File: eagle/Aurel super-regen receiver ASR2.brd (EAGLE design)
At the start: 43.2 x 25.4 mm, 15 parts, among them T1 BF247B

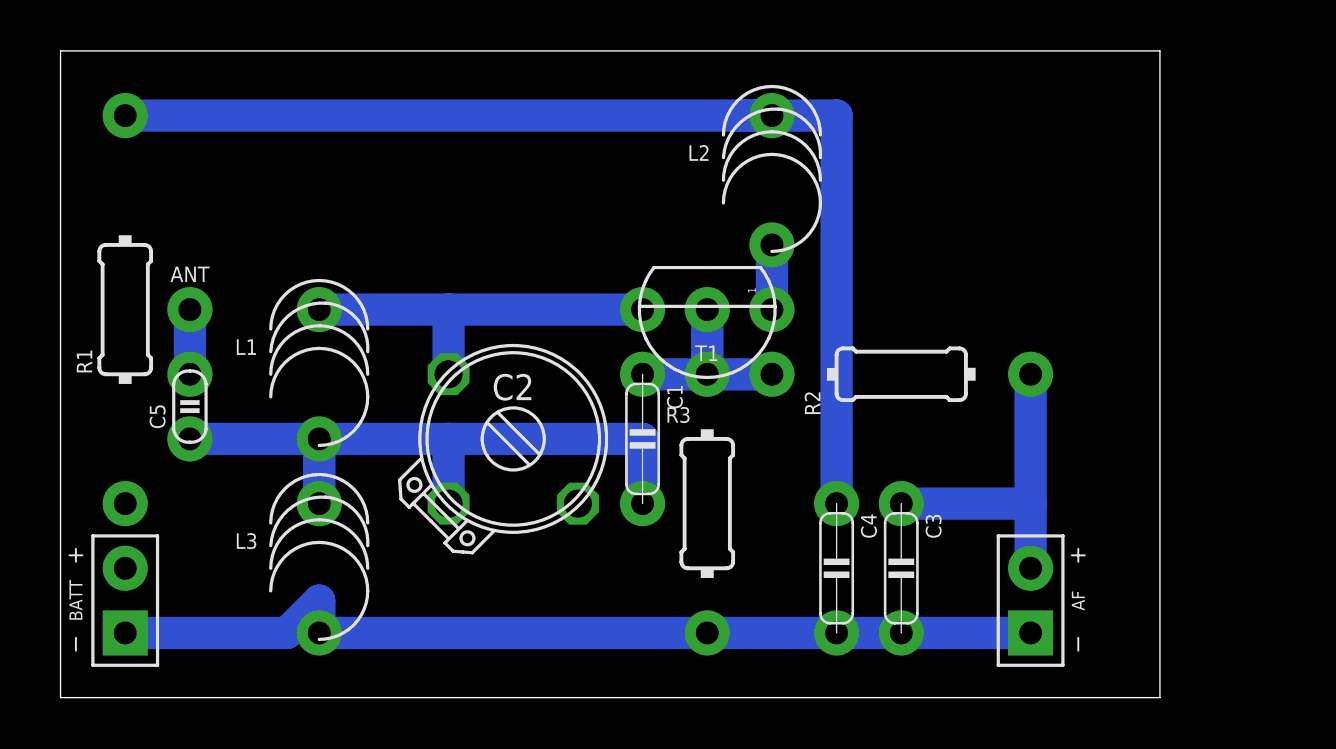
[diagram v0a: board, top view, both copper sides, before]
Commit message: ...
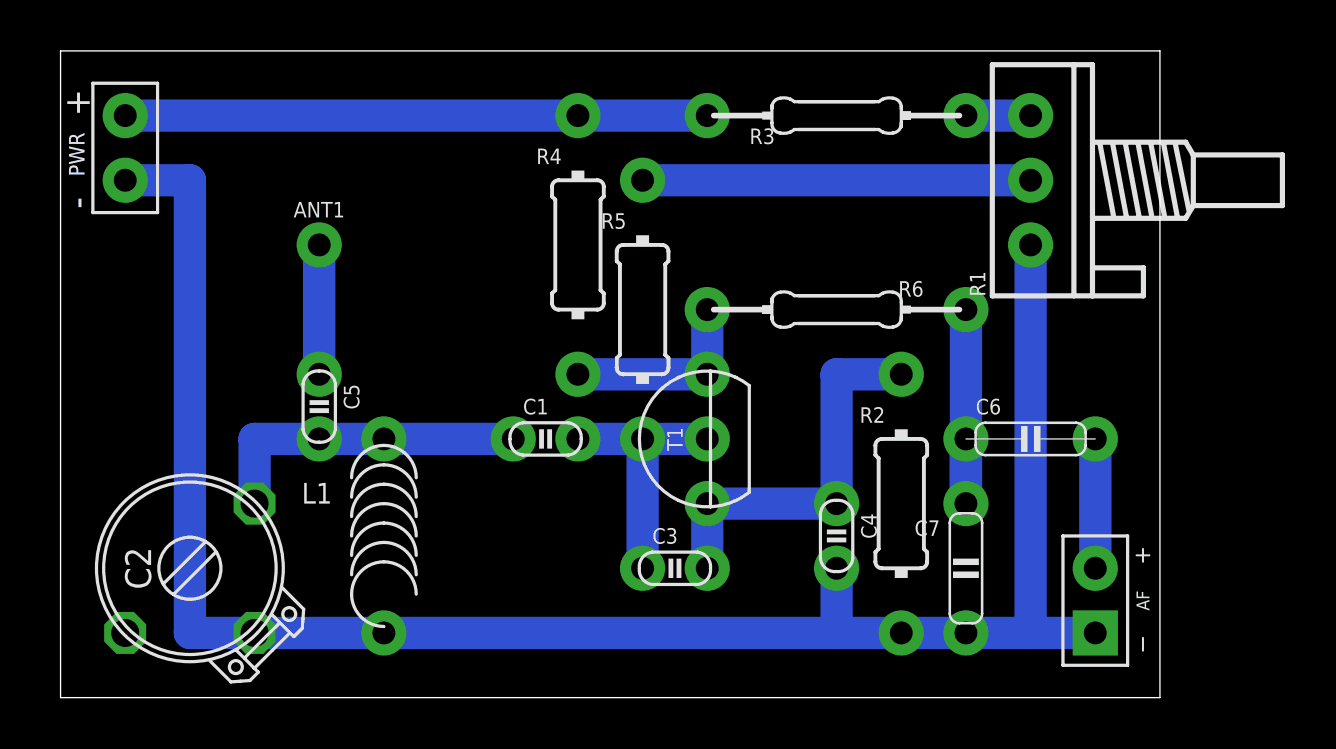
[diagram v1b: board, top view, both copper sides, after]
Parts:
- removed ANT: ANT, pad:SPAD
- removed BATT: SPAD+--+, pad:SPAD-+
- removed L2: 73nH, l:L-04-5/5V-C
- removed L3: 40nH, l:L-04-5/5V-C
- added ANT1: ANT, pad:SPAD
- added C6: 47nF, c:C050-020X044
- added C7: 1nF, c:C050-020X044/V
- added R4, R5: 1kΩ, r:0204/10-V
- added R6: 1kΩ, r:0204/10
- added S2: (no value), pad:PWR-L
- AF: value SPAD+-+- -> (none)
- C1: value 5nF -> 5pF; device c:C050-020X044 -> c:C025-015X024
- C2: value 33pF -> 2 - 20pF
- C3: value 6.8nF -> 33pF; device c:C050-020X044 -> c:C025-015X024
- C4: value 100nF -> 10pF; device c:C050-020X044 -> c:C025-015X024
- C5: value 15p -> 1pF
- L1: value 100nH -> 200nH; device l:L-04-5/5V-C -> l:L-04/7-V
- R1: value 150 -> 10kΩ; device r:0204/15-V -> r:POT
- R2: value 10k -> 1kΩ
- R3: value 3.3k -> 10kΩ; device r:0204/10-V -> r:0204/10
- T1: value BF247B -> 2N2222; device t:TO92 -> t:TO92-EBC
- moved R1 35.9 mm to (38.1, 20.3), turned to 90 degrees
- moved R3 16.1 mm to (30.5, 22.9), turned to 180 degrees
- moved C2 13.7 mm to (5.08, 5.08), turned to 90 degrees
- moved C3 8.89 mm to (24.1, 5.08), turned to 0 degrees
- moved L1 6.84 mm to (12.7, 6.35)
- moved C5 5.08 mm to (10.2, 11.4), turned to 270 degrees
- moved T1 5.08 mm to (25.4, 10.2), turned to 180 degrees
- moved R2 5.08 mm to (33.0, 7.62), turned to 0 degrees
- moved C1 3.81 mm to (19.1, 10.2), turned to 0 degrees
- moved AF 2.54 mm to (40.6, 3.81)
- moved C4 1.27 mm to (30.5, 6.35)
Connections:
- removed net N$4: AF.2, C3.1, R2.2
- new net N$10: C6.1, C7.1, R6.2
- new net N$11: AF.2, C6.2
- new net VCC: R3.2, R4.1, S2.2
- net GND: now also C2.2, C7.2, L1.2, R1.A, R2.2, S2.1; no longer BATT.1, C3.2, L3.1, R3.2
- net N$1: now also ANT1.1, C5.1; no longer C2.1, L1.2, T1.3
- net N$2: now also C1.1, C2.3, C5.2; no longer C1.2, C2.2, C5.1, L3.2
- net N$3: now also C1.2, C3.1, R5.2, T1.B; no longer C4.1, L2.2, R1.1
- net N$5: now also C3.2, C4.1, T1.E; no longer C1.1, R3.1, T1.2
- net N$6: now also R4.2, R6.1, T1.C; no longer L2.1, T1.1
- net N$7: now also R1.S, R5.1; no longer BATT.2, R1.2
- net N$8: now also R1.E, R3.1; no longer ANT.1, C5.2
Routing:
- net GND: track 37.4 -> 73.7 mm
- net N$3: track 44.5 -> 10.2 mm
- net VCC: track 0.00 -> 22.9 mm
- net N$7: track 0.00 -> 15.2 mm
- net N$4: track 12.7 -> 0.00 mm
- net N$2: track 25.4 -> 12.7 mm
- net N$10: track 0.00 -> 10.2 mm
- net N$1: track 15.2 -> 5.08 mm
- net N$5: track 7.62 -> 15.2 mm
- net N$11: track 0.00 -> 5.08 mm
- net N$6: track 2.54 -> 7.62 mm
